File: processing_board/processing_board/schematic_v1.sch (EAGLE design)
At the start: 28 parts, among them Q1 BSS138, Q2 BSS138

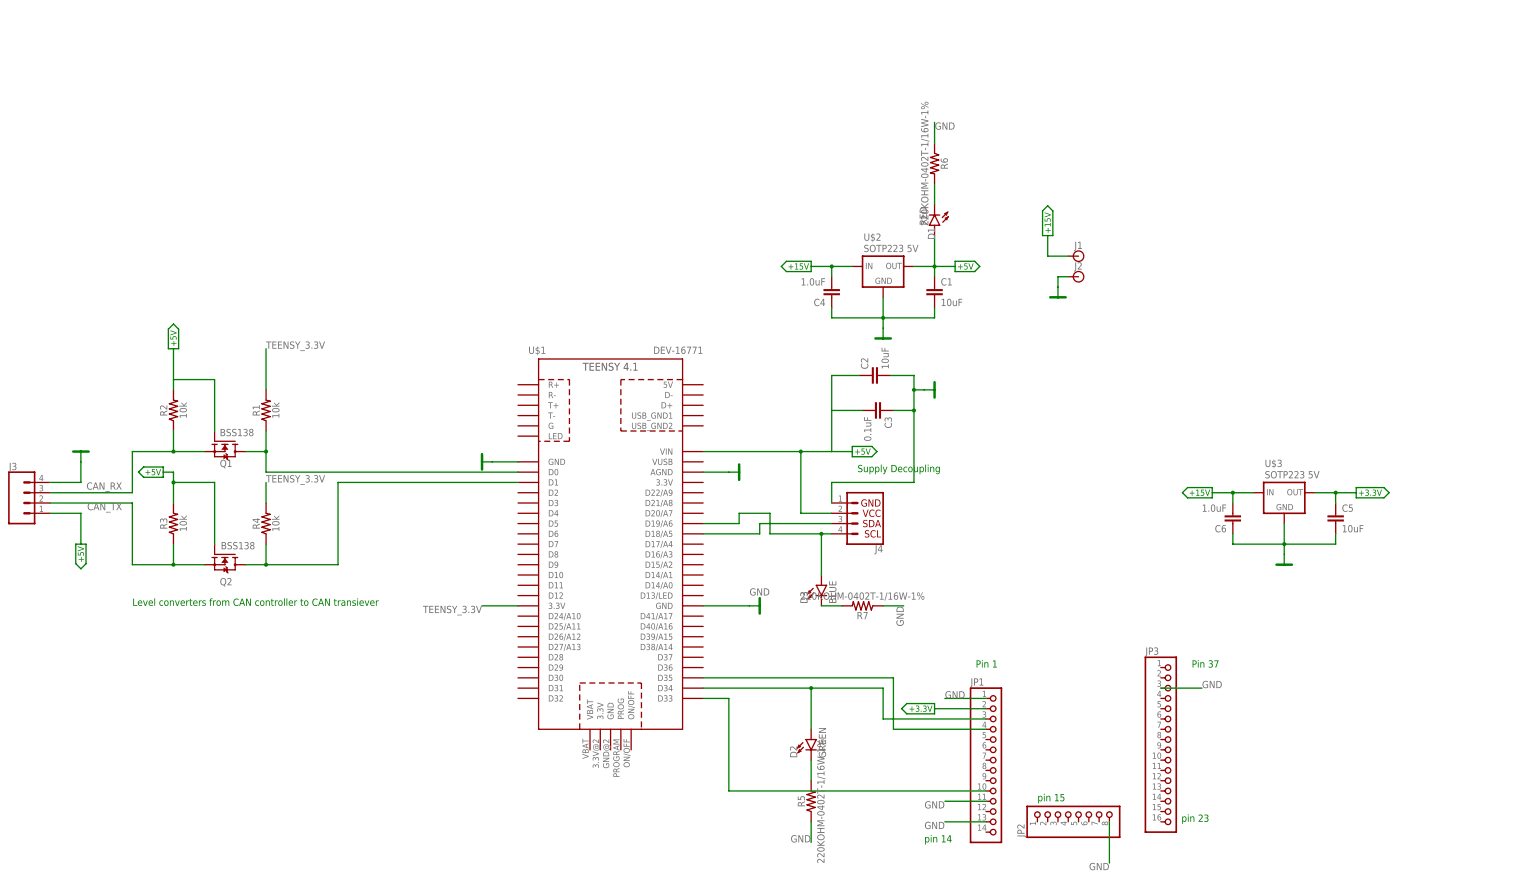
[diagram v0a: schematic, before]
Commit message: updated schematic
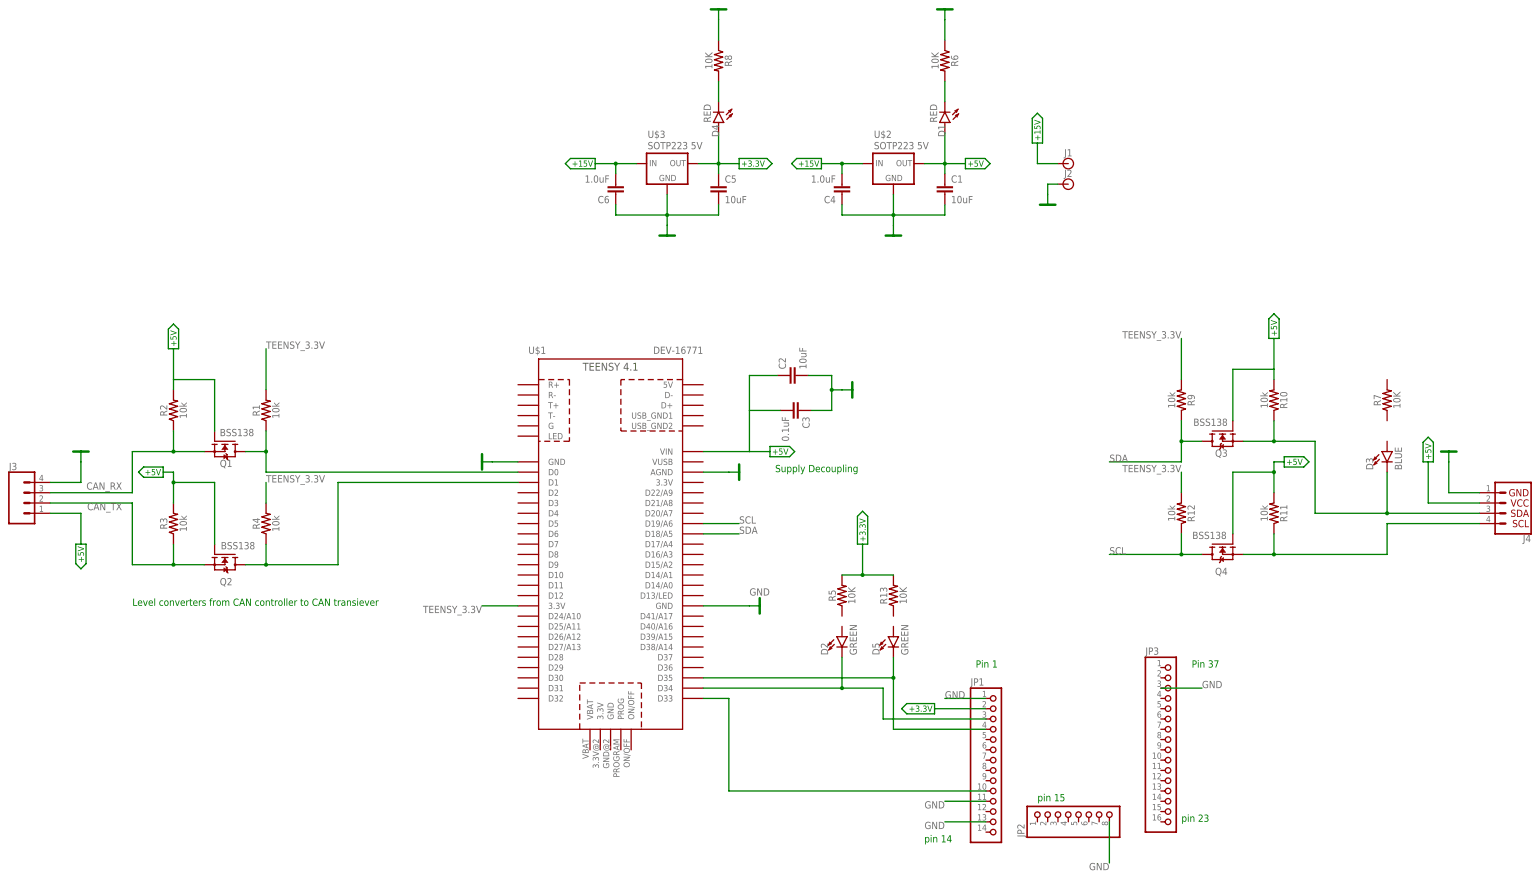
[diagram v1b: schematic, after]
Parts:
- added D4: RED, SparkFun-LED:LED-RED0603
- added D5: GREEN, SparkFun-LED:LED-GREEN0603
- added Q3, Q4: BSS138, BSS138:BSS138
- added R10, R11, R12, R9: 10k, SparkFun-Resistors:10KOHM-0603-1/10W-1%
- added R13, R8: 10K, SparkFun-Resistors:220KOHM-0402T-1/16W-1%
- R5, R6, R7: value 220KOHM-0402T-1/16W-1% -> 10K
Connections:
- removed net N$4: D2.C, R5.2
- removed net N$5: J4.3, U$1.D18/A5
- removed net N$6: D3.A, J4.4, U$1.D19/A6
- removed net N$8: D3.C, R7.2
- new net +5V1: D4.A
- new net CAN_RX1: D3.C, J4.3, Q3.S, R10.1
- new net CAN_TX1: J4.4, Q4.S, R11.1
- new net N$10: D4.C, R8.2
- new net SCL: Q4.D, R12.1, U$1.D19/A6
- new net SDA: Q3.D, R9.1, U$1.D18/A5
- net +3.3V: now also R13.2, R5.2
- net +5V: now also Q3.G, Q4.G, R10.2, R11.2
- net GND: now also R8.1; no longer R5.1, R7.1
- net N$1: now also D5.C
- net N$2: now also D2.C; no longer D2.A
- net TEENSY_3.3V: now also R12.2, R9.2
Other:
- moved on the sheet: C1, C2, C3, C4, C5, C6, D1, D2, D3, J1, J2, J4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
